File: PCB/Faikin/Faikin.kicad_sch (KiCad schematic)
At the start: 28 parts, among them J1 1x5, J2 TC2030-USB-NL-DS, J3 Reset, Q1 BSS138PS, U2 ESP32-S3-MINI-1, U3 MD8942

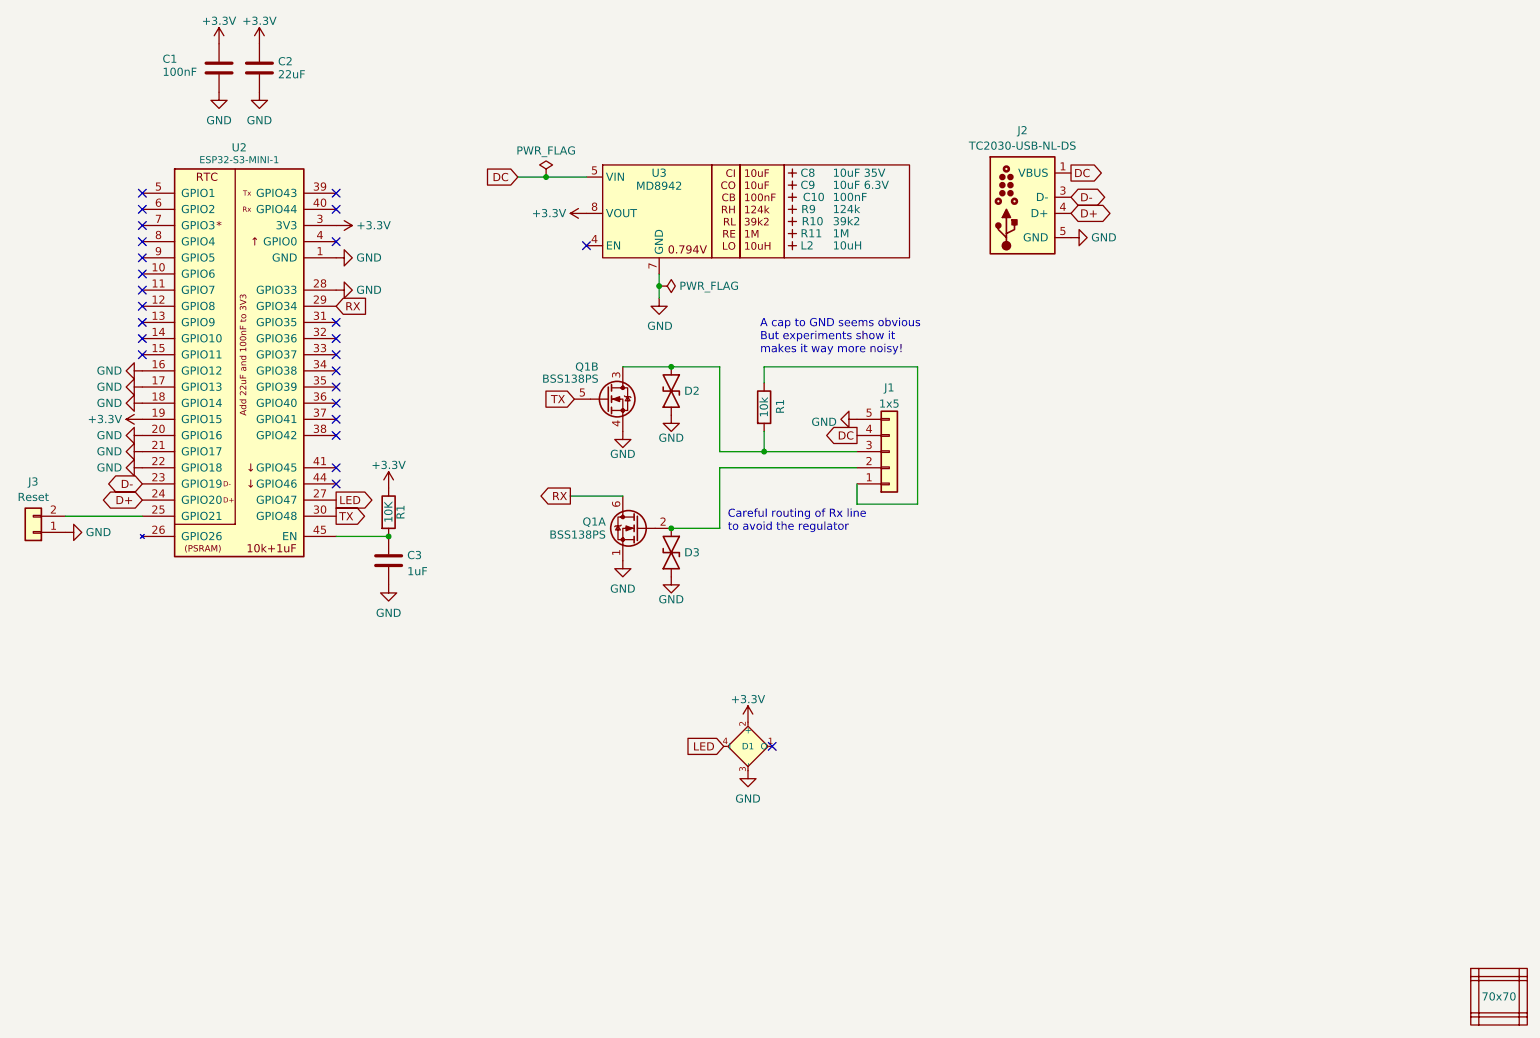
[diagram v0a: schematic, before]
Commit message: PCb tweaks
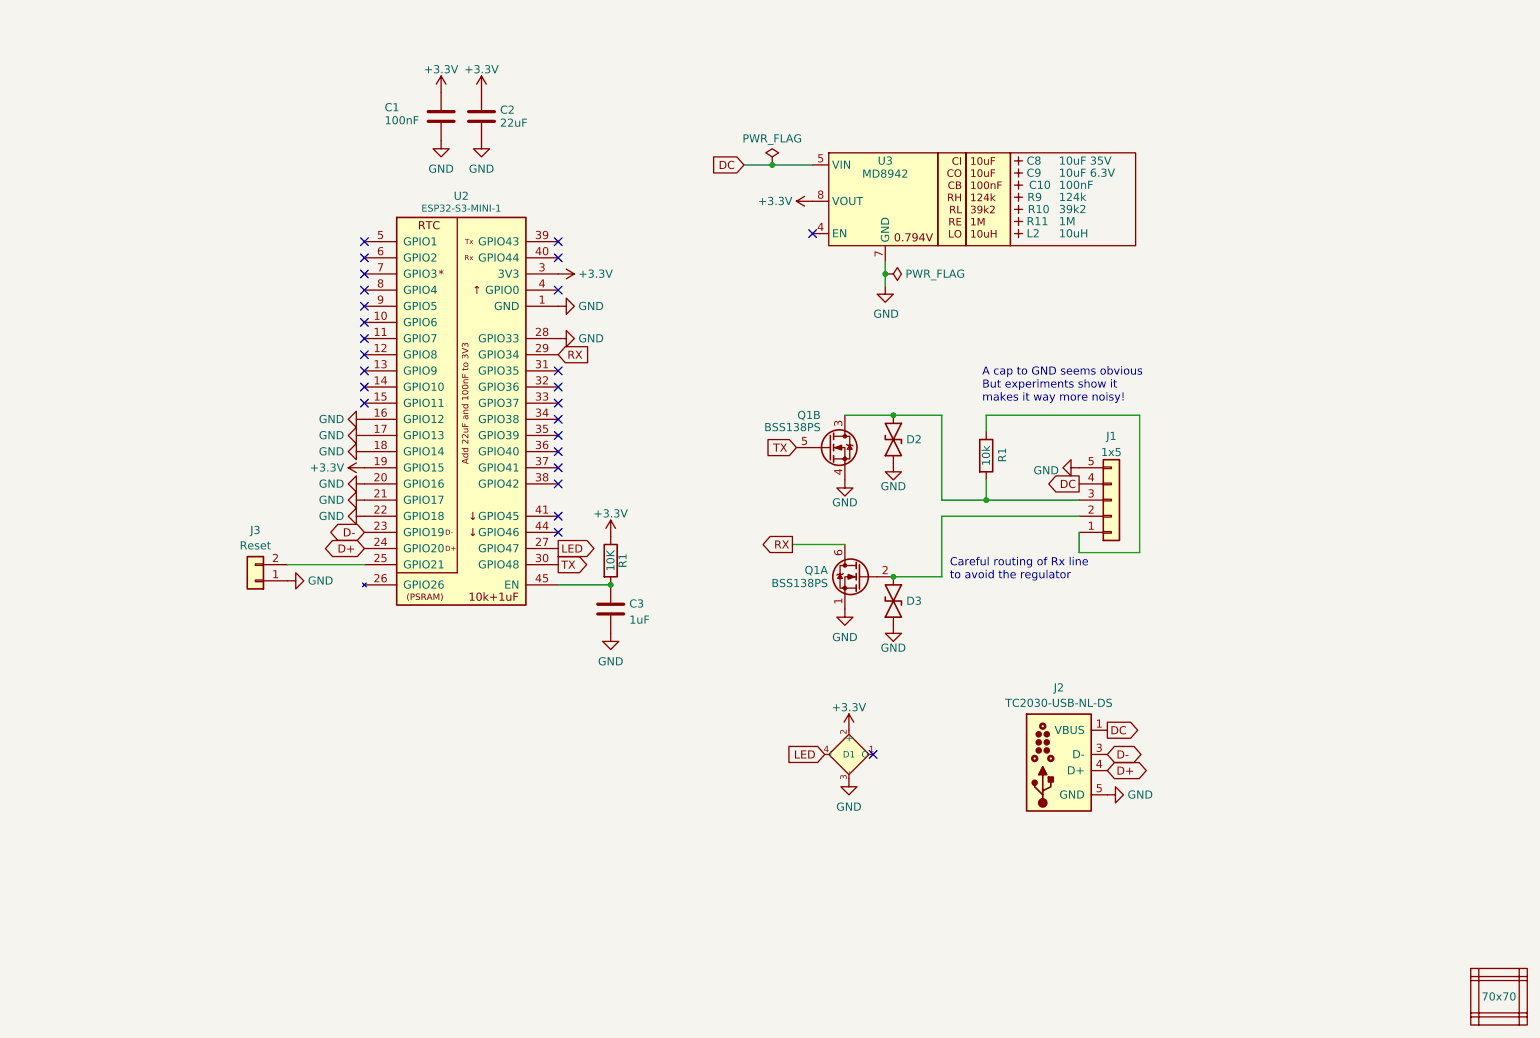
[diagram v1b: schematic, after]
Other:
- moved on the sheet: C1, C10, C2, C3, C8, C9, D1, D2, D3, J1, J2, J3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
